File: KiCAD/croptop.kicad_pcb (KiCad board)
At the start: 4 copper layers, 115.6 x 45.7 mm, 269 parts, among them J1 PICKit Header, J2 USB_A, J3 5V USB, J4 4-1734839-0, J5 Terminal Block, J6 DNP, J7 DNP, SW1 BTNA, SW2 BTNA, U1 PIC32MX795F512L, U10 AD7799, U11 74HCT125D, U12 Si7006-A20, U13 UCAM-M8Q, U14 W25N01GV, U15 LIS3DH, U16 PUSBM5V5X4, U17 DT6250-06MR-13, U18 PUSBM5V5X4, U2 REG71055, U3 FAN5333BSX, U4 MIC23050, U5 TC1014, U6 FT812Q, U8 74HCT125D, U9 DRV8872, Y1 CXO, Y2 12MHz

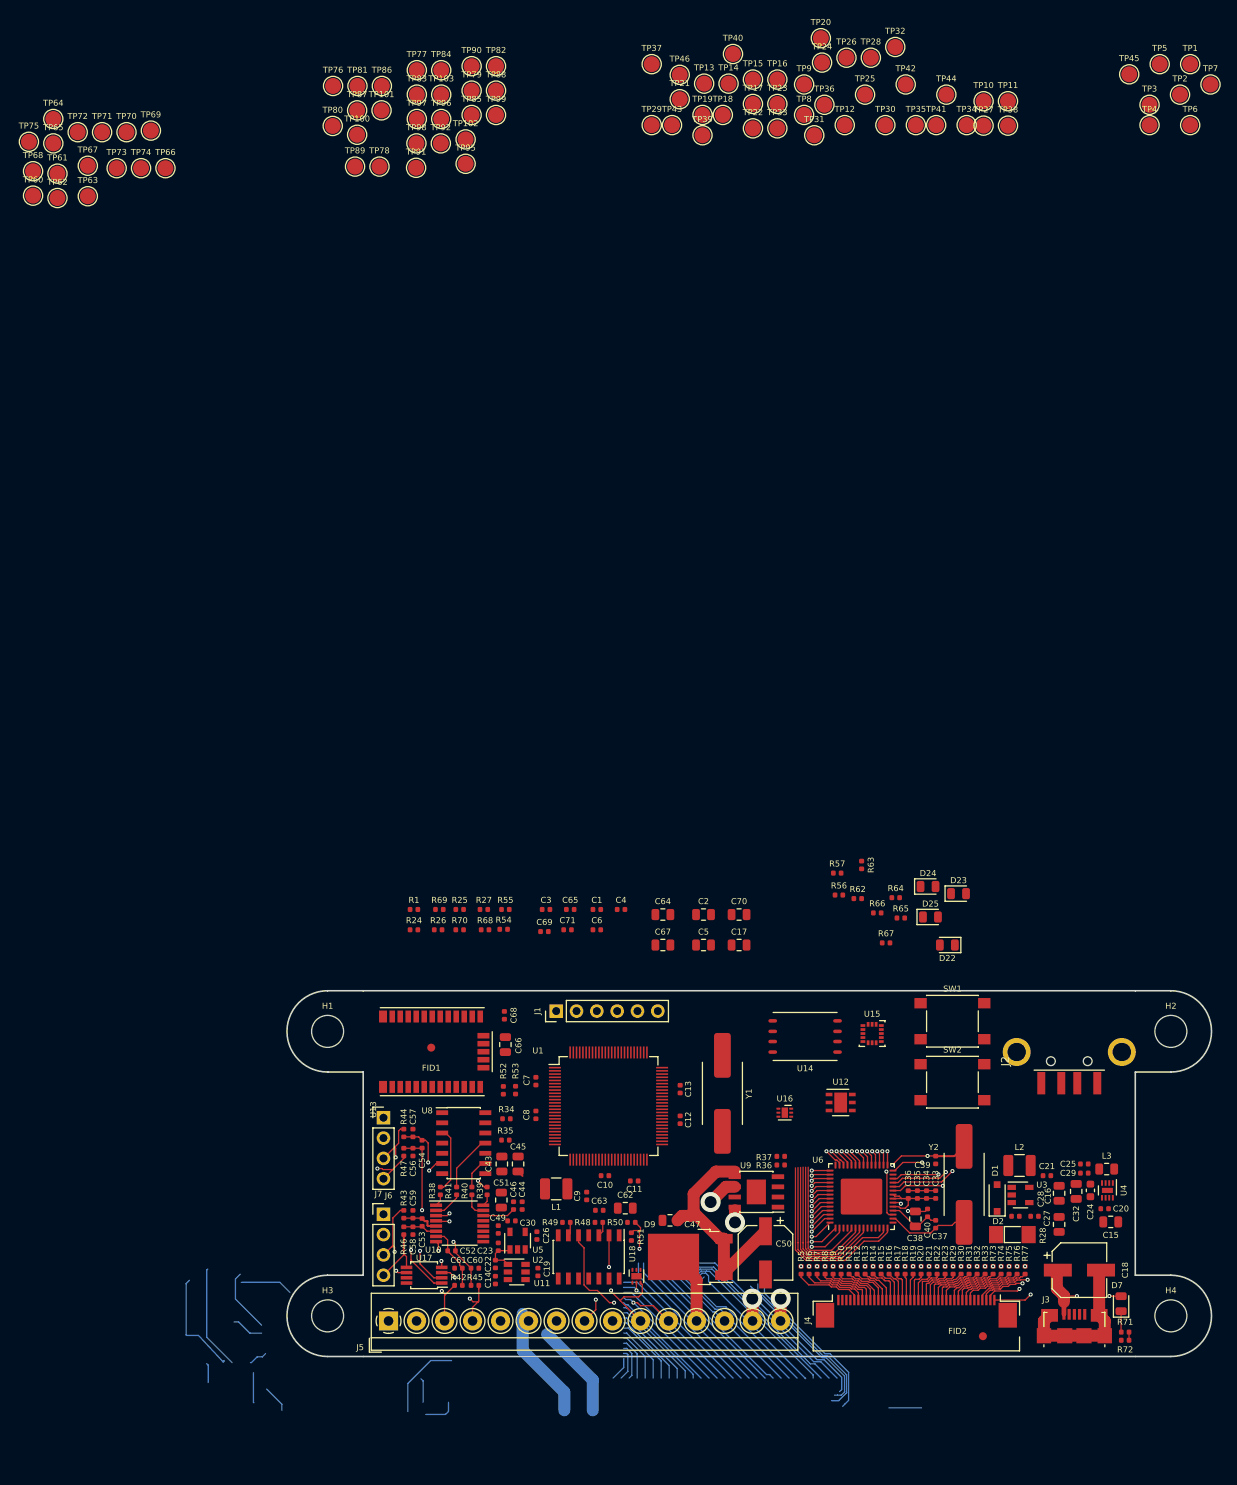
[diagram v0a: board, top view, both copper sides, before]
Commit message: Finished working board
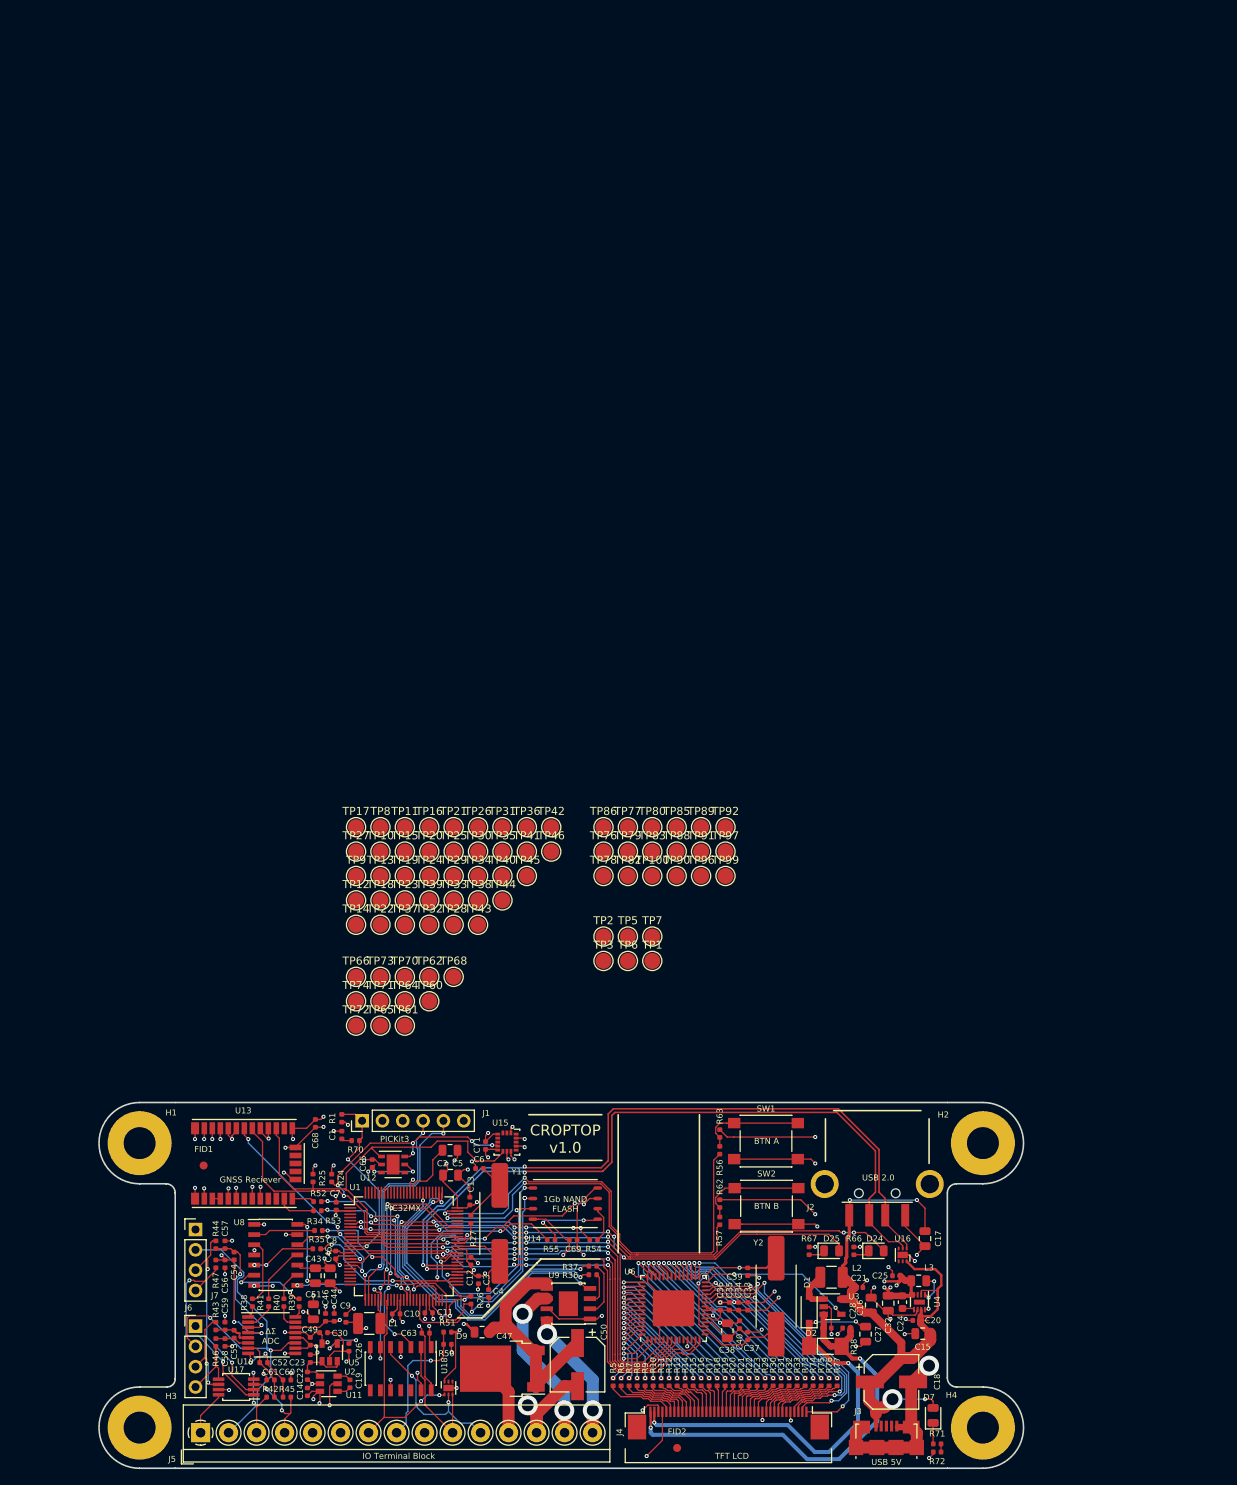
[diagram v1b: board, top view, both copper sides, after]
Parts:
- removed C29: 1uF, Capacitor_SMD:C_0402_1005Metric
- removed C62, C64, C66, C67, C70: 10uF, Capacitor_SMD:C_0805_2012Metric
- removed D22: LED4, LED_SMD:LED_0805_2012Metric
- removed D23: LED3, LED_SMD:LED_0805_2012Metric
- removed R48, R49, R68, R69: 10, Resistor_SMD:R_0402_1005Metric
- removed R64, R65: 60, Resistor_SMD:R_0402_1005Metric
- removed TP101, TP102, TP103, TP4, TP63, TP67, TP69, TP75, TP81, TP84, TP87, TP95, TP98: TestPoint_Alt, TestPoint:TestPoint_Pad_D2.0mm
- H1, H2, H3, H4: footprint MountingHole:MountingHole_4mm -> MountingHole:MountingHole_4mm_Pad
- moved TP1 130.7 mm to (135.8, 78.8)
- moved TP5 127.7 mm to (132.8, 75.8)
- moved TP2 127.5 mm to (129.7, 75.8)
- moved TP7 127.3 mm to (135.8, 75.8)
- moved TP3 126.9 mm to (129.7, 78.8)
- moved TP6 125.9 mm to (132.8, 78.8)
- moved TP45 125.3 mm to (120.2, 68.2)
- moved TP32 124.2 mm to (108.0, 74.3)
- moved TP10 120.3 mm to (101.9, 65.2)
- moved TP28 120.3 mm to (111.0, 74.3)
- moved TP27 119.9 mm to (98.8, 65.2)
- moved TP64 118.7 mm to (104.9, 83.9)
- moved TP11 118.0 mm to (104.9, 62.1)
- moved TP65 117.6 mm to (101.9, 86.9)
- moved TP38 117.3 mm to (114.1, 71.3)
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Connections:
- C10 pad 1: LIN_VDD -> DVDD
- C11 pad 1: LIN_VDD -> DVDD
- C12 pad 1: LIN_VDD -> DVDD
- C13 pad 1: LIN_VDD -> DVDD
- C14 pad 1: VBUS -> DVDD_UNREG
- C15 pad 1: VBUS -> DVDD_UNREG
- C16 pad 1: VBUS -> DVDD_UNREG
- C17 pad 1: VBUS -> DVDD_UNREG
- C18 pad 1: VBUS -> DVDD_UNREG
- C20 pad 1: VBUS -> DVDD_UNREG
- C21 pad 1: VBUS -> DVDD_UNREG
- C24 pad 2: LIN_VDD -> DVDD
- C25 pad 1: LIN_VDD -> DVDD
- C3 pad 1: LIN_VDD -> DVDD
- C32 pad 1: LIN_VDD -> DVDD
- C33 pad 1: LIN_VDD -> DVDD
- C34 pad 1: LIN_VDD -> DVDD
- C35 pad 1: LIN_VDD -> DVDD
- C36 pad 1: LIN_VDD -> DVDD
- C43 pad 1: LIN_VDD -> DVDD
- C44 pad 1: LIN_VDD -> DVDD
- C45 pad 1: LIN_VDD -> DVDD
- C46 pad 1: LIN_VDD -> DVDD
- C5 pad 1: LIN_VDD -> DVDD
- C63 pad 1: LIN_VDD -> DVDD
- C65 pad 1: LIN_VDD -> DVDD
- C68 pad 1: LIN_VDD -> DVDD
- C69 pad 1: LIN_VDD -> DVDD
- C7 pad 1: LIN_VDD -> DVDD
- C71 pad 1: LIN_VDD -> DVDD
- C8 pad 1: LIN_VDD -> DVDD
- C9 pad 1: LIN_VDD -> DVDD
- D7 pad 2: VBUS -> DVDD_UNREG
- J1 pad 2: LIN_VDD -> DVDD
- J1 pad 4: Net-(J1-Pad4) -> PKT_PGED
- J1 pad 5: Net-(J1-Pad5) -> PKT_PGEC
- J2 pad 1: VBUS -> DVDD_UNREG
- J3 pad 1: VBUS -> DVDD_UNREG
- J4 pad 4: LIN_VDD -> DVDD
- J5 pad 5: LIN_VDD -> DVDD
- L1 pad 1: LIN_VDD -> DVDD
- L2 pad 2: VBUS -> DVDD_UNREG
- L3 pad 1: LIN_VDD -> DVDD
- R1 pad 1: LIN_VDD -> DVDD
- R24 pad 1: LIN_VDD -> DVDD
- R25 pad 1: LIN_VDD -> DVDD
- R50 pad 1: LIN_VDD -> DVDD
- R51 pad 2: VBUS -> DVDD_UNREG
- SW1 pad 2: Net-(R56-Pad2) -> DVDD
- SW2 pad 2: Net-(R57-Pad2) -> DVDD
- TP1 pad 1: LIN_VDD -> DVDD
- TP5 pad 1: VBUS -> DVDD_UNREG
- U1 pad 16: LIN_VDD -> DVDD
- U1 pad 19: LCD_INT -> GPS_INT
- U1 pad 2: LIN_VDD -> DVDD
- U1 pad 20: BTN_A -> Net-(U1-Pad20)
- U1 pad 21: BTN_B -> Net-(U1-Pad21)
- U1 pad 32: GPS_INT -> Net-(U1-Pad32)
- U1 pad 37: LIN_VDD -> DVDD
- U1 pad 46: LIN_VDD -> DVDD
- U1 pad 54: VBUS -> DVDD_UNREG
- U1 pad 55: LIN_VDD -> DVDD
- U1 pad 62: LIN_VDD -> DVDD
- U1 pad 73: Net-(U1-Pad73) -> BTN_B
- U1 pad 74: Net-(U1-Pad74) -> BTN_A
- U1 pad 8: LED_C -> Net-(U1-Pad8)
- U1 pad 86: LIN_VDD -> DVDD
- U1 pad 9: LED_D -> Net-(U1-Pad9)
- U10 pad 14: LIN_VDD -> DVDD
- U11 pad 14: LIN_VDD -> DVDD
- U11 pad 3: Net-(R48-Pad1) -> ROT_Y1
- U11 pad 6: Net-(R49-Pad1) -> ROT_Y2
- U12 pad 5: LIN_VDD -> DVDD
- U13 pad 1: LIN_VDD -> DVDD
- U13 pad 8: LIN_VDD -> DVDD
- U13 pad 9: LIN_VDD -> DVDD
- U14 pad 8: LIN_VDD -> DVDD
- U15 pad 1: LIN_VDD -> DVDD
- U15 pad 14: LIN_VDD -> DVDD
- U15 pad 7: LIN_VDD -> DVDD
- U15 pad 8: LIN_VDD -> DVDD
- U16 pad 6: VBUS -> DVDD_UNREG
- U18 pad 6: LIN_VDD -> DVDD_UNREG
- U2 pad 3: VBUS -> DVDD_UNREG
- U2 pad 5: VBUS -> DVDD_UNREG
- U3 pad 5: VBUS -> DVDD_UNREG
- U4 pad 2: VBUS -> DVDD_UNREG
- U4 pad 4: LIN_VDD -> DVDD
- U4 pad 7: VBUS -> DVDD_UNREG
- U6 pad 11: LIN_VDD -> DVDD
- U6 pad 19: LIN_VDD -> DVDD
- U6 pad 21: LIN_VDD -> DVDD
- U6 pad 22: LIN_VDD -> DVDD
- U8 pad 14: LIN_VDD -> DVDD
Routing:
- net DRV_GND: track 65.4 -> 260.9 mm, vias 0 -> 91
- net DVDD: track 0.00 -> 148.8 mm, vias 0 -> 38
- net DVDD_UNREG: track 0.00 -> 116.2 mm, vias 0 -> 9
- net USB_D+: track 0.00 -> 92.2 mm, vias 0 -> 2
- net USB_D-: track 0.00 -> 92.1 mm, vias 0 -> 2
- net LED_B: track 0.00 -> 71.0 mm, vias 0 -> 8
- net LED_A: track 0.00 -> 66.7 mm, vias 0 -> 8
- net SCL: track 0.00 -> 64.4 mm, vias 0 -> 6
- net SDA: track 0.00 -> 61.4 mm
- net BTN_A: track 0.00 -> 57.6 mm, vias 0 -> 2
- net LCD_CATHODE: track 0.00 -> 54.5 mm, vias 0 -> 2
- net LCD_ANODE: track 0.00 -> 53.9 mm, vias 0 -> 4
- net SCLK: track 0.00 -> 52.9 mm, vias 0 -> 10
- net ADC_GND: track 0.00 -> 51.7 mm, vias 0 -> 2
- net BTN_B: track 0.00 -> 48.6 mm, vias 0 -> 2
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- added copper zone on Vdd.Cu, net ADC_VDD
- added copper zone on Gnd.Cu, net DRV_GND
- added copper zone on Vdd.Cu, net DVDD
- added copper zone on Vdd.Cu, net DVDD_UNREG
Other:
- outline, holes or cut-outs redrawn
- board text added: "1Gb NAND FLASH"
- board text added: "BOARD MODEL:"
- board text added: "BTN A"
- board text added: "BTN B"
- board text added: "BY KENNEDY CAISLEY & RYAN DONAHUE"
- board text added: "CROPTOP v1.0"
- board text added: "DATA ACQUISITION PLATFORM"
- board text added: "DESIGNED AT THE UNIVERSITY OF IDAHO"
- board text added: "FOR AGRICULTURE RESEARCH"
- board text added: "GNSS Reciever"
- board text added: "IO Terminal Block"
- board text added: "PIC32MX"
- board text added: "PICKit3"
- board text added: "TFT LCD"
- board text added: "USB 2.0"
- board text added: "USB 5V"
- board text added: "ΔΣ ADC"
